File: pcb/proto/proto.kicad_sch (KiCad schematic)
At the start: 1 part

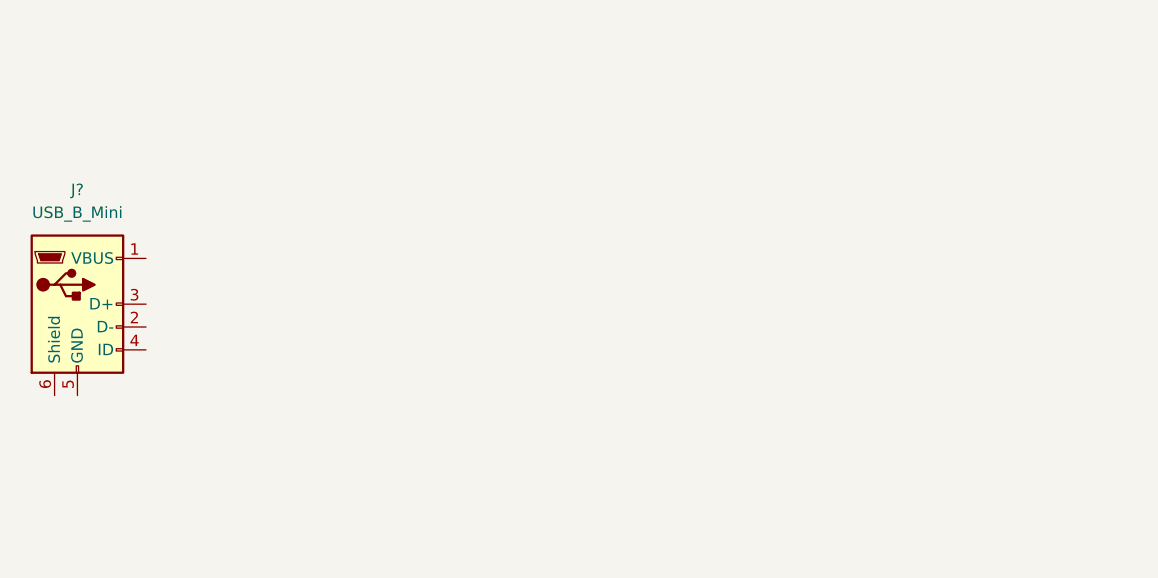
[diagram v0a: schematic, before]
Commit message: Signed-off-by: Dmitry Ponyatov <ponyatov@example.com>
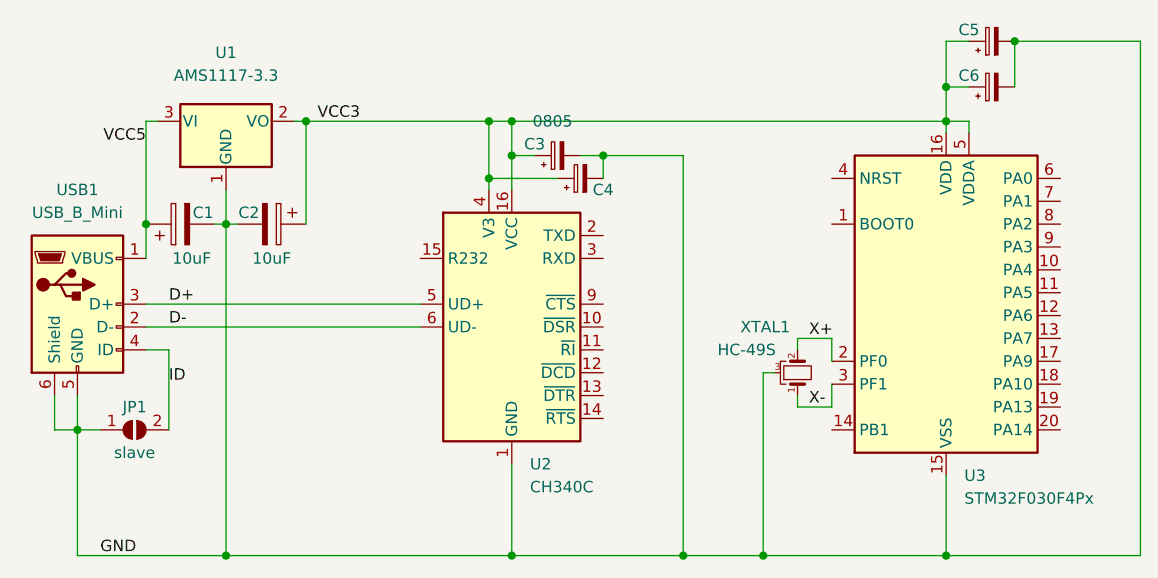
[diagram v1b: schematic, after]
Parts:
- added C1, C2: 10uF, Capacitor_SMD:C_1206_3216Metric_Pad1.33x1.80mm_HandSolder, symbol Device:C_Polarized
- added C3: 0805, Capacitor_SMD:C_0805_2012Metric_Pad1.18x1.45mm_HandSolder, symbol Device:C_Polarized_Small
- added C4: 0603, Capacitor_SMD:C_0603_1608Metric_Pad1.08x0.95mm_HandSolder, symbol Device:C_Polarized_Small
- added C5, C6: C_Polarized_Small, Capacitor_SMD:C_0402_1005Metric_Pad0.74x0.62mm_HandSolder, symbol Device:C_Polarized_Small
- added JP1: slave, Resistor_SMD:R_0201_0603Metric, symbol Jumper:SolderJumper_2_Open
- added U1: AMS1117-3.3, Package_TO_SOT_SMD:SOT-223-3_TabPin2, symbol Regulator_Linear:AMS1117-3.3
- added U2: CH340C, Package_SO:SOIC-16_3.9x9.9mm_P1.27mm, symbol Interface_USB:CH340C
- added U3: STM32F030F4Px, Package_SO:TSSOP-20_4.4x6.5mm_P0.65mm, symbol MCU_ST_STM32F0:STM32F030F4Px
- added XTAL1: HC-49S, crystal:Crystal_HC49-2P_mill, symbol crystal:HC-49S
- USB1: renamed from J?; footprint Connector_USB:USB3_Micro-B_Connfly_DS1104-01 -> Connector_USB:USB_Mini-B_DS1104
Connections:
- net VCC5: now reaches USB1.1 (VBUS)
- net VCC5: now also C1.1, U1.3 (VI)
- net D-: now reaches USB1.2 (D-)
- net D-: now also U2.6 (UD-)
- net D+: now reaches USB1.3 (D+)
- net D+: now also U2.5 (UD+)
- net ID: now reaches USB1.4 (ID)
- net ID: now also JP1.2 (B)
- net GND: now reaches USB1.5 (GND)
- net GND: now also USB1.6 (Shield), C1.2, C2.2, C3.2, C4.2, C5.2, C6.2, JP1.1 (A), U1.1 (GND), U2.1 (GND), U3.15 (VSS), XTAL1.3
- new net VCC3: C2.1, C3.1, C4.1, C5.1, C6.1, U1.2 (VO), U2.16 (VCC), U2.4 (V3), U3.16 (VDD), U3.5 (VDDA)
- new net X+: U3.2 (PF0), XTAL1.2
- new net X-: U3.3 (PF1), XTAL1.1
